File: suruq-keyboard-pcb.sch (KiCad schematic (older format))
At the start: 20 parts

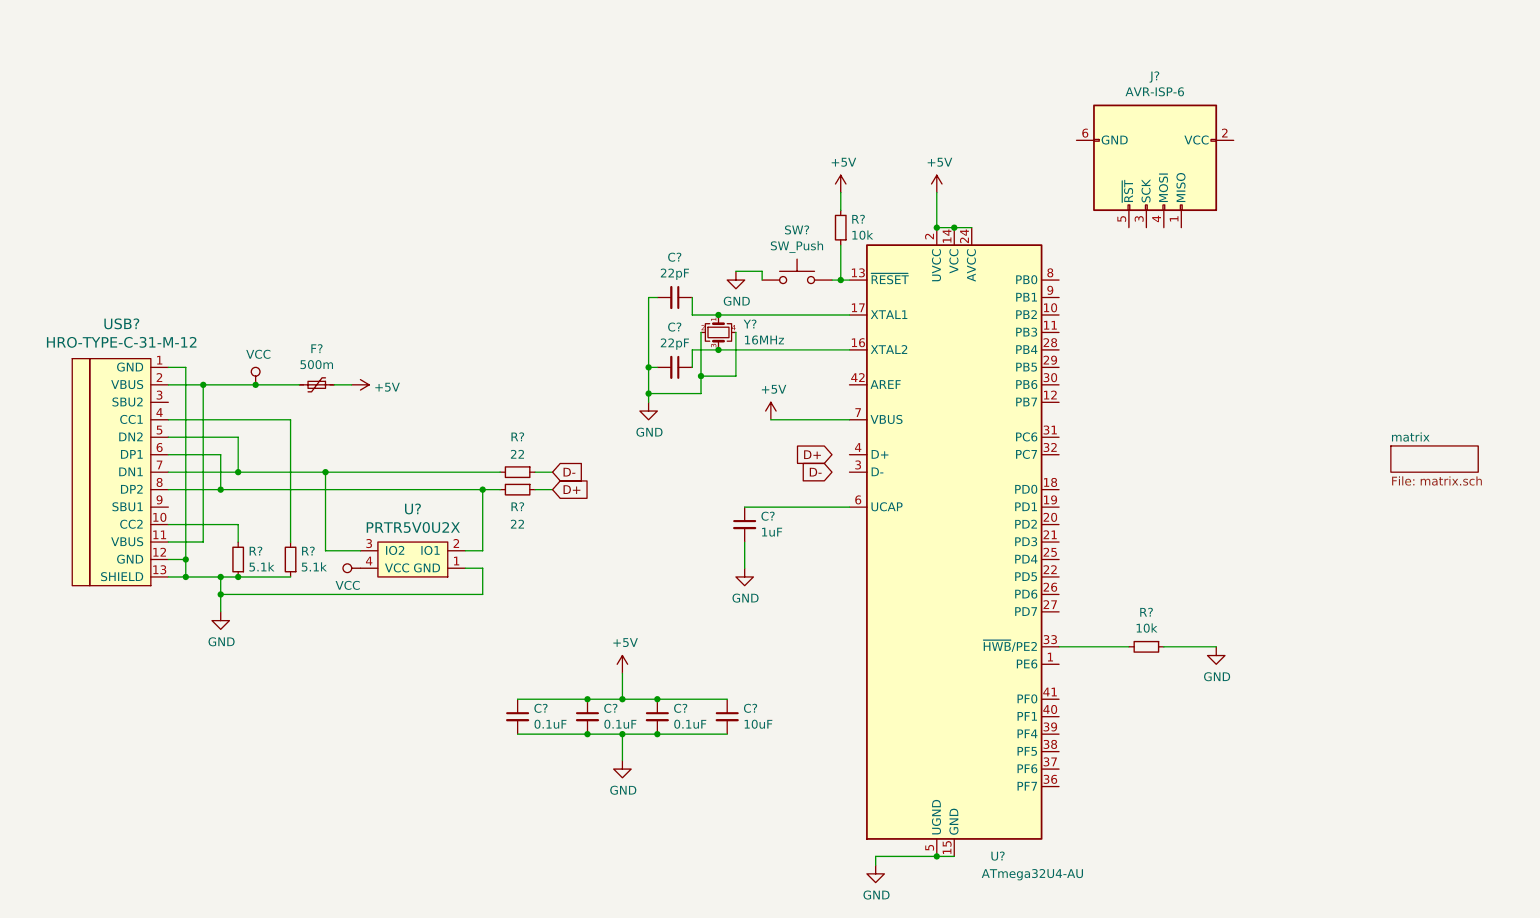
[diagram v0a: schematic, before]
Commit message: pcb layout routing WIP
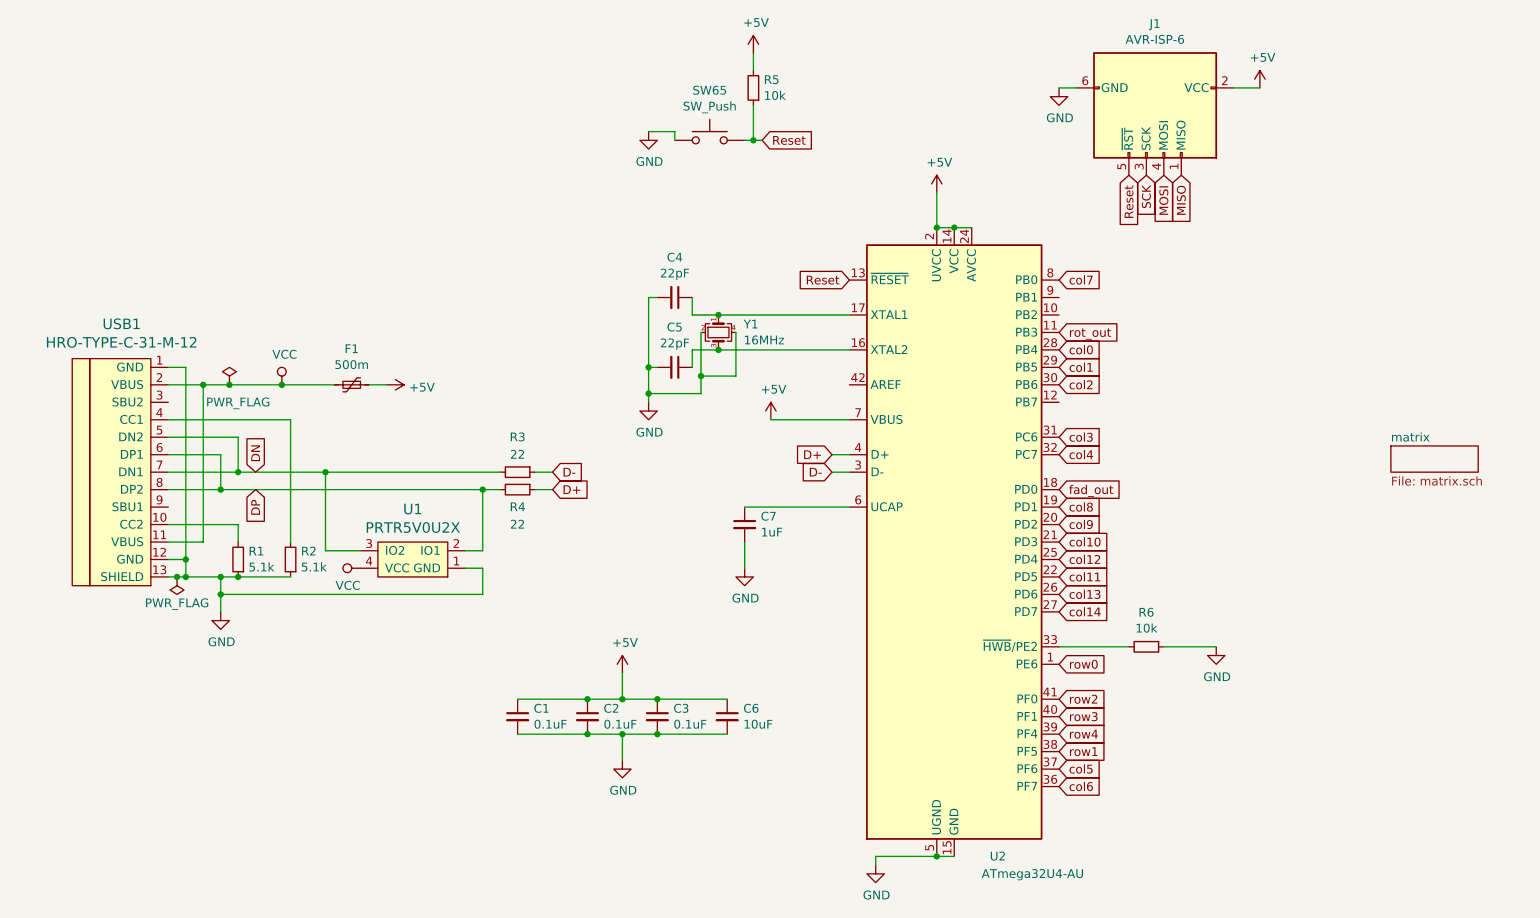
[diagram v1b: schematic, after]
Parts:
- C1, C2, C3, C4, C5, C6, C7: renamed from C?; footprint (none) -> Capacitor_SMD:C_0805_2012Metric_Pad1.15x1.40mm_HandSolder
- F1: renamed from F?; footprint (none) -> Fuse:Fuse_1206_3216Metric_Pad1.42x1.75mm_HandSolder
- J1: renamed from J?; footprint (none) -> random-keyboard-parts:Reset_Pretty-Mask
- R1, R2, R3, R4, R5, R6: renamed from R?; footprint (none) -> Resistor_SMD:R_0805_2012Metric_Pad1.15x1.40mm_HandSolder
- SW65: renamed from SW?; footprint (none) -> Button_Switch_Keyboard:SW_Cherry_MX_1.00u_PCB
- U1: renamed from U?; footprint (none) -> random-keyboard-parts:SOT143B
- USB1: renamed from USB?; footprint (none) -> Type-C:HRO-TYPE-C-31-M-12-HandSoldering
- Y1: renamed from Y?; footprint (none) -> Crystal:Crystal_SMD_3225-4Pin_3.2x2.5mm_HandSoldering
- gave numbers to parts that had none: 1
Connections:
- net +5V: now also J1.2 (VCC)
- net D+: now also U2.4 (D+)
- net D-: now also U2.3 (D-)
- net GND: now also J1.6 (GND)
- net row0: now reaches U2.1 (PE6)
- net rot_out: now reaches U2.11 (PB3)
- net Reset: now reaches R5.1, SW65.2, U2.13 (~RESET)
- net Reset: now also J1.5 (~RST)
- net fad_out: now reaches U2.18 (PD0)
- net col8: now reaches U2.19 (PD1)
- net col9: now reaches U2.20 (PD2)
- net col10: now reaches U2.21 (PD3)
- net col11: now reaches U2.22 (PD5)
- net col12: now reaches U2.25 (PD4)
- net col13: now reaches U2.26 (PD6)
- net col14: now reaches U2.27 (PD7)
- net col0: now reaches U2.28 (PB4)
- net col1: now reaches U2.29 (PB5)
- net col2: now reaches U2.30 (PB6)
- net col3: now reaches U2.31 (PC6)
- net col4: now reaches U2.32 (PC7)
- net col6: now reaches U2.36 (PF7)
- net col5: now reaches U2.37 (PF6)
- net row1: now reaches U2.38 (PF5)
- net row4: now reaches U2.39 (PF4)
- net row3: now reaches U2.40 (PF1)
- net row2: now reaches U2.41 (PF0)
- net col7: now reaches U2.8 (PB0)
- net DN: now reaches R3.2, U1.3 (IO2), USB1.5 (DN2), USB1.7 (DN1)
- net DP: now reaches R4.2, U1.2 (IO1), USB1.6 (DP1), USB1.8 (DP2)
- net MISO: now reaches J1.1 (MISO)
- net SCK: now reaches J1.3 (SCK)
- net MOSI: now reaches J1.4 (MOSI)
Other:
- moved on the sheet: F1, J1, R5, SW65
